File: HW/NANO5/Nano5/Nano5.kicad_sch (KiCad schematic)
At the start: 131 parts, among them J1 Screw_Terminal_01x03, J10 Screw_Terminal_01x03, J11 Screw_Terminal_01x03, J12 Screw_Terminal_01x02, J13 Conn_02x04_Counter_Clockwise, J14 Conn_02x04_Counter_Clockwise, J15 Conn_02x03_Counter_Clockwise, J16 Conn_01x02, J17 Conn_01x02, J2 Screw_Terminal_01x03, J3 Screw_Terminal_01x03, J4 Screw_Terminal_01x03, J5 Screw_Terminal_01x02, J6 Screw_Terminal_01x02, J7 Screw_Terminal_01x02, J8 Screw_Terminal_01x03, J9 Screw_Terminal_01x03, K1 SANYOU_SRD_Form_C, K2 SANYOU_SRD_Form_C, K3 SANYOU_SRD_Form_C, K4 SANYOU_SRD_Form_C, K5 SANYOU_SRD_Form_C, K6 SANYOU_SRD_Form_C, Q1 MMBT3904, Q2 MMBT3904, Q3 MMBT3904, Q4 MMBT3904, Q5 MMBT3904, Q6 MMBT3904, U1 ATmega328P-A, U10 ESP-12E, U11 M24C02-RMN, U12 ST485EBDR, U13 DS1307Z+, U14 MP1584, U15 LM358, U16 AP1117-33, U2 LTV-817S, U3 LTV-817S, U4 LTV-817S, U5 LTV-817S, U6 LTV-817S, U7 LTV-817S, U8 LTV-817S, U9 LTV-817S, Y1 Crystal_Small

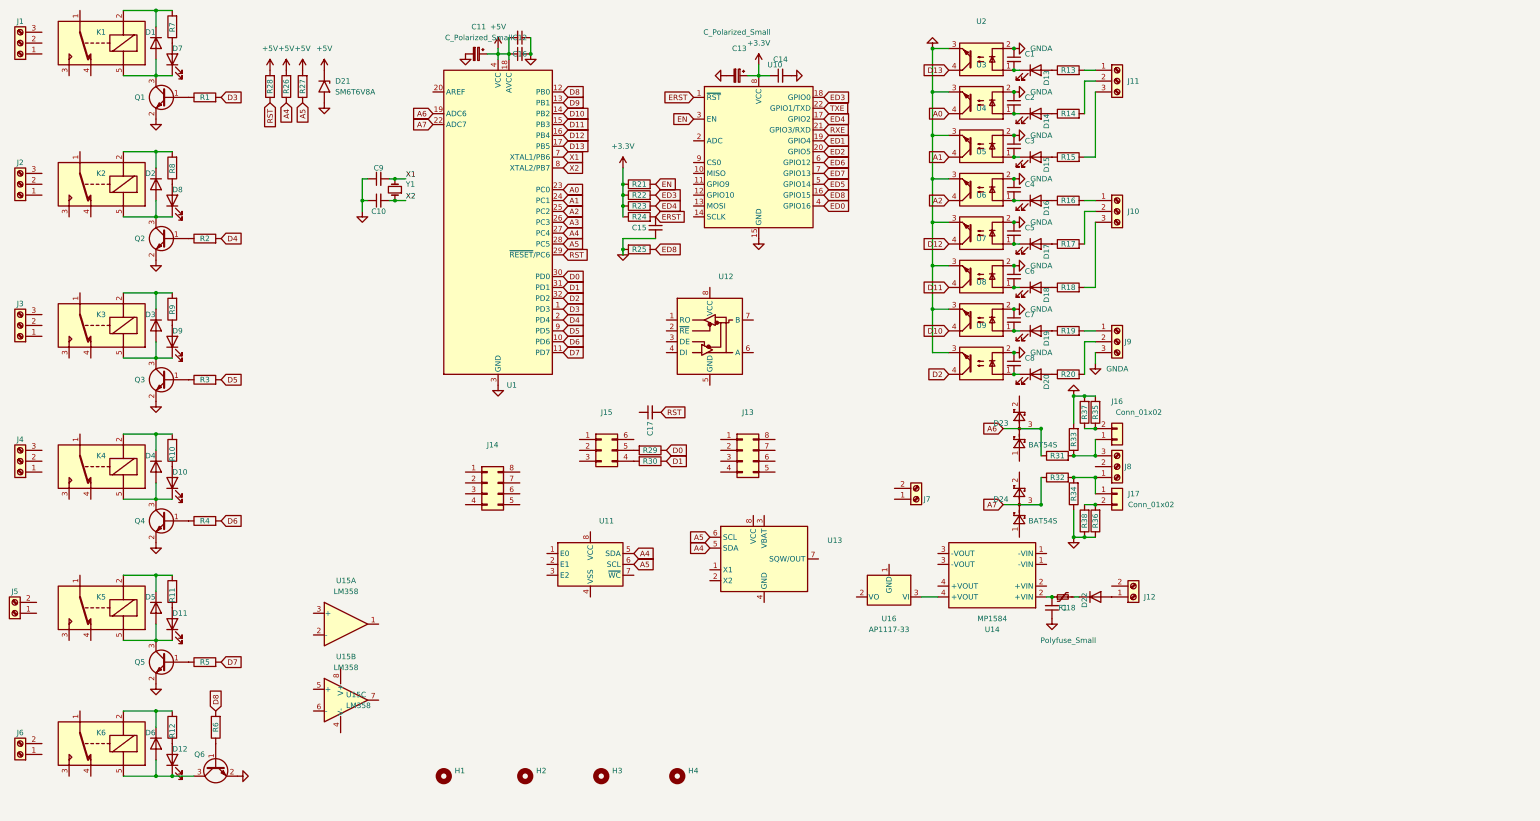
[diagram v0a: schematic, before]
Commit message: MAJOR UPDATE
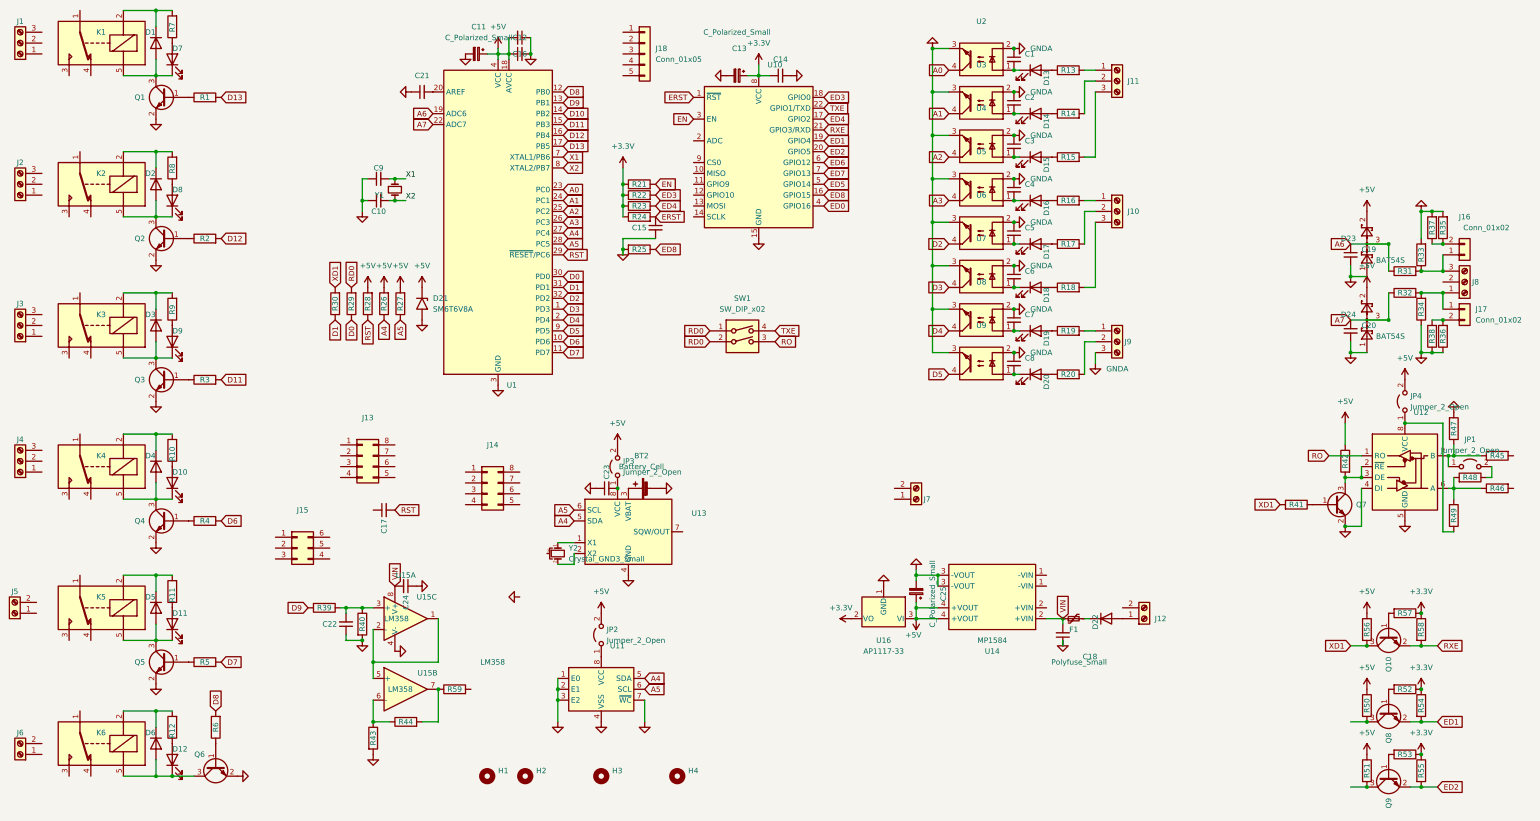
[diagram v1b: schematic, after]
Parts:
- added BT2: Battery_Cell, Battery:BatteryHolder_Keystone_1058_1x2032, symbol Device:Battery_Cell
- added C19, C20: C_Small, Capacitor_SMD:C_0805_2012Metric, symbol Device:C_Small
- added C21, C22, C23, C24: 100nF, Capacitor_SMD:C_0805_2012Metric, symbol Device:C_Small
- added C25: C_Polarized_Small, Capacitor_SMD:CP_Elec_4x3.9, symbol Device:C_Polarized_Small
- added J18: Conn_01x05, Connector_PinHeader_2.54mm:PinHeader_1x05_P2.54mm_Vertical, symbol Connector_Generic:Conn_01x05
- added JP1: Jumper_2_Open, Jumper:SolderJumper-2_P1.3mm_Open_RoundedPad1.0x1.5mm, symbol Jumper:Jumper_2_Open
- added JP2, JP3, JP4: Jumper_2_Open, Jumper:SolderJumper-2_P1.3mm_Bridged_RoundedPad1.0x1.5mm, symbol Jumper:Jumper_2_Open
- added Q10, Q7, Q8, Q9: MMBT3904, Package_TO_SOT_SMD:SOT-23, symbol Transistor_BJT:MMBT3904
- added R39, R40, R41, R42, R43, R44, R45, R46, R47, R48, R49, R50, R51, R52, R53, R54, R55, R56, R57, R58, R59: R, Resistor_SMD:R_0805_2012Metric, symbol Device:R
- added SW1: SW_DIP_x02, Button_Switch_SMD:SW_DIP_SPSTx02_Slide_6.7x6.64mm_W8.61mm_P2.54mm_LowProfile, symbol Switch:SW_DIP_x02
- added Y2: Crystal_GND3_Small, Crystal:Crystal_SMD_FrontierElectronics_FM206, symbol Device:Crystal_GND3_Small
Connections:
- net +3V3: now also U16.2 (VO), R52.1, R53.1, R54.1, R55.1, R57.1, R58.1
- net +5V: now also D23.2, D24.2, U14.4 (+VOUT), U16.3 (VI), C25.1, JP2.2 (B), JP3.2 (B), JP4.2 (B), R42.1, R50.1, R51.1, R56.1
- net A0: now also U2.4; no longer U3.4
- net A1: now also U3.4; no longer U4.4
- net A2: now also U4.4; no longer U5.4
- net A3: now also U5.4
- net A6: now also C19.1
- net A7: now also C20.1
- net D10: no longer U8.4
- net D11: now also R3.2; no longer U7.4
- net D12: now also R2.2; no longer U6.4
- net D13: now also R1.2; no longer U2.4
- net D2: now also U6.4; no longer U9.4
- net D3: now also U7.4; no longer R1.2
- net D4: now also U8.4; no longer R2.2
- net D5: now also U9.4; no longer R3.2
- net D9: now also R39.2
- net ED1: now also Q8.2 (E), R54.2
- net ED2: now also Q9.2 (E), R55.2
- net GND: now also D23.1, D24.1, U11.1 (E0), U11.2 (E1), U11.3 (E2), U11.4 (VSS), U11.7 (~{WC}), U12.4 (DI), U12.5 (GND), U13.4 (GND), U14.3 (-VOUT), U15.4 (V-), U16.1 (GND), BT2.2 (-), C19.2, C20.2, C21.1, C22.1, C23.1, C24.1, C25.2, Q7.2 (E), R40.2, R43.2, R47.2
- net RXE: now also Q10.2 (E), R58.2
- net TXE: now also SW1.4
- net X1: now also Y1.1; no longer Y1.2
- net X2: now also Y1.2; no longer Y1.1
- net at J15.5 (Pin_5): no longer R29.2
- net RO: now reaches U12.1 (RO)
- net RO: now also SW1.3
- net at U12.2 (~{RE}): now also U12.3 (DE), Q7.3 (C), R42.2
- net at U12.6 (A): now also R46.1, R48.2, R49.2
- net at U12.7 (B): now also JP1.1 (A), R45.1, R47.1
- net at U12.8 (VCC): now also JP4.1 (A), R49.1
- net VIN: now reaches C18.2, F1.1, U14.2 (+VIN)
- net VIN: now also U15.8 (V+), C24.2
- net at U15.1: now also U15.2 (-), U15.5 (+)
- net at U15.3 (+): now also C22.2, R39.1, R40.1
- net at J15.4 (Pin_4): no longer R30.2
- net at U15.6 (-): now also R43.1, R44.1
- net at U15.7: now also R44.2, R59.1
- net at U13.1 (X1): now also Y2.1
- net at U13.2 (X2): now also Y2.2
- net at U13.3 (VBAT): now also BT2.1 (+)
- net at U13.8 (VCC): now also C23.2, JP3.1 (A)
- net at U11.8 (VCC): now also JP2.1 (A)
- net at U1.20 (AREF): now also C21.2
- new net: Q9.1 (B), R53.2
- new net: Q9.3 (C), R51.2
- new net: Q10.1 (B), R57.2
- new net: JP1.2 (B), R48.1
- new net: Q7.1 (B), R41.1
- new net: Q8.1 (B), R52.2
- new net: Q8.3 (C), R50.2
- new net RD0: R29.2, SW1.1, SW1.2
- new net XD1: Q10.3 (C), R30.2, R41.2, R56.2
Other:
- moved on the sheet: C17, C18, D21, D22, D23, D24, F1, H1, J12, J13, J15, J16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
